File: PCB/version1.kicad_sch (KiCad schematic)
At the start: 21 parts, among them J1 USB_C_Receptacle_USB2.0_16P, SW1 SW_SPST, SW2 SW_SPST, SW3 RotaryEncoder_Switch, U1 STM32F072CBTx, U2 XC6206PxxxMR

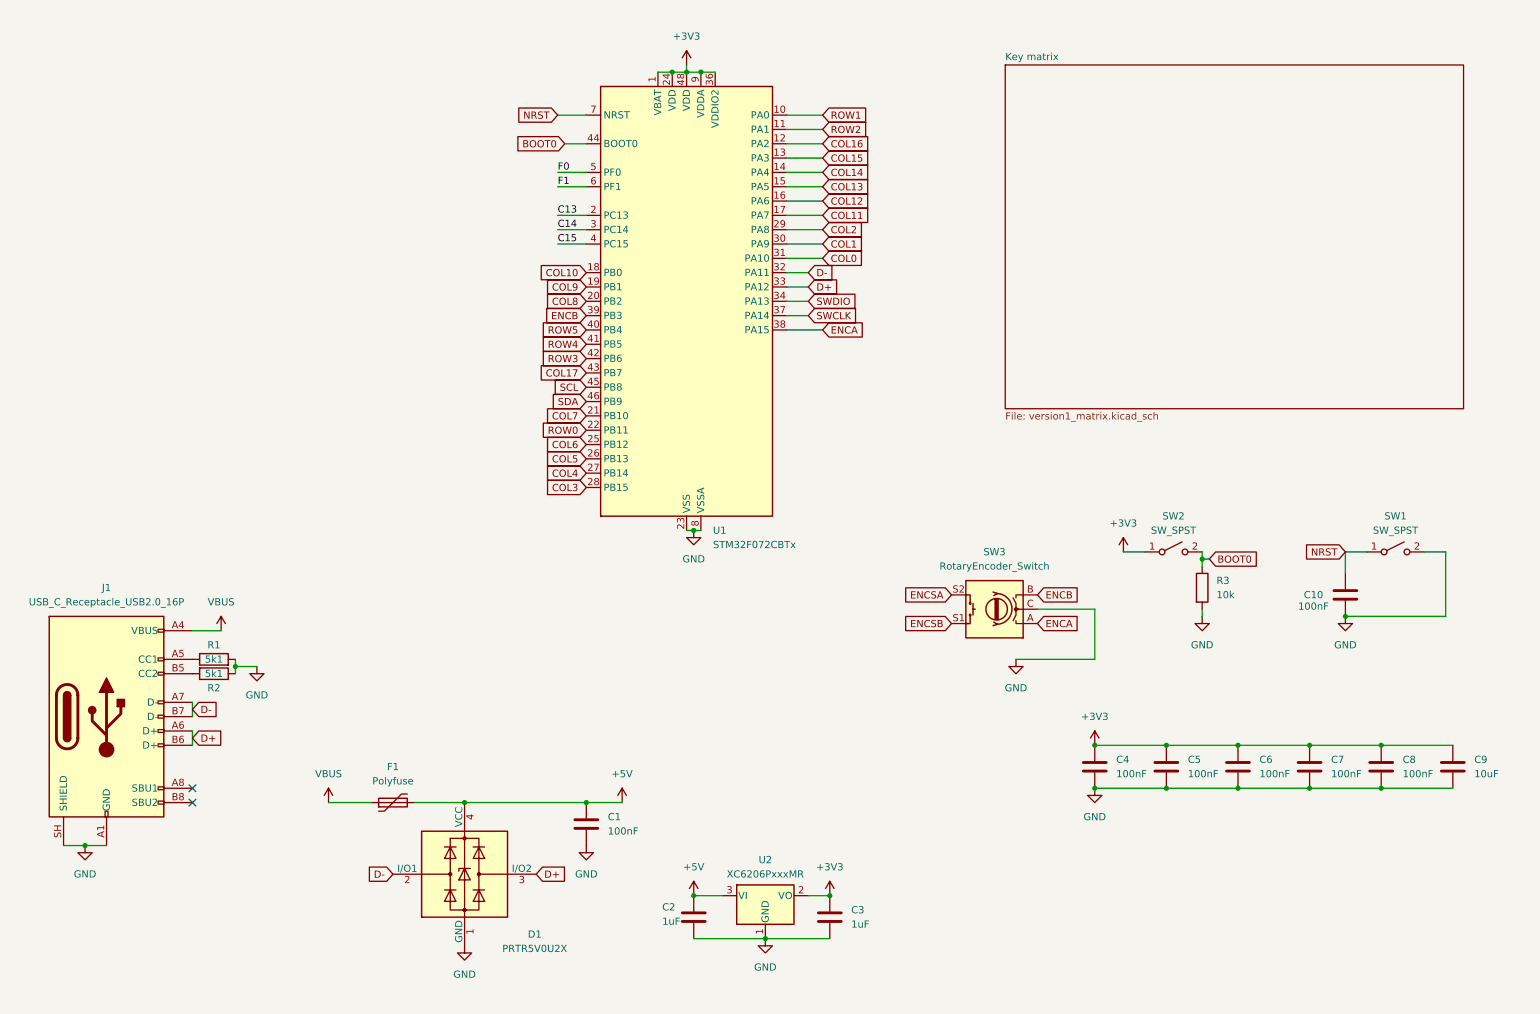
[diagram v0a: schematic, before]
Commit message: Updated schematic
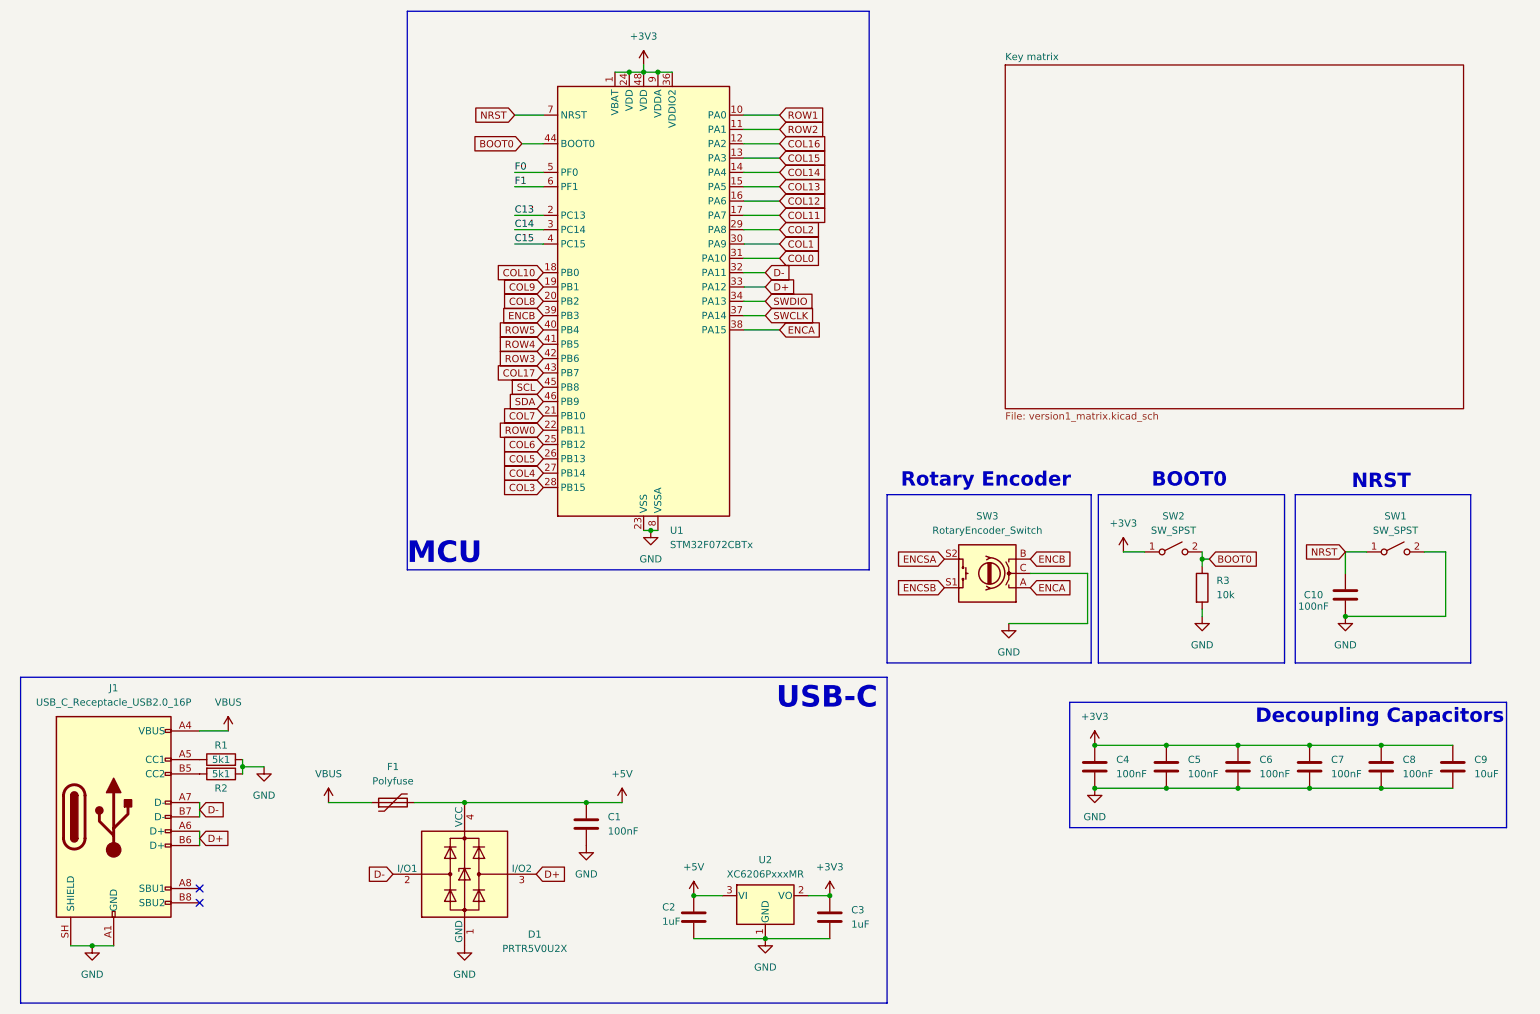
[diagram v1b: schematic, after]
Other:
- note added: "BOOT0"
- note added: "Decoupling Capacitors"
- note added: "MCU"
- note added: "NRST"
- note added: "Rotary Encoder"
- note added: "USB-C"
- moved on the sheet: J1, R1, R2, SW3, U1

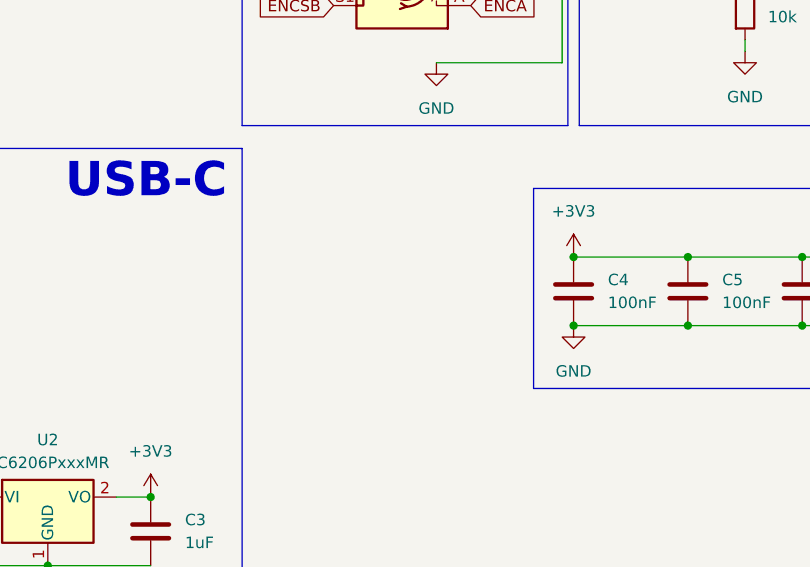
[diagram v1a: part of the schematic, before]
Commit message: Updated PCB files
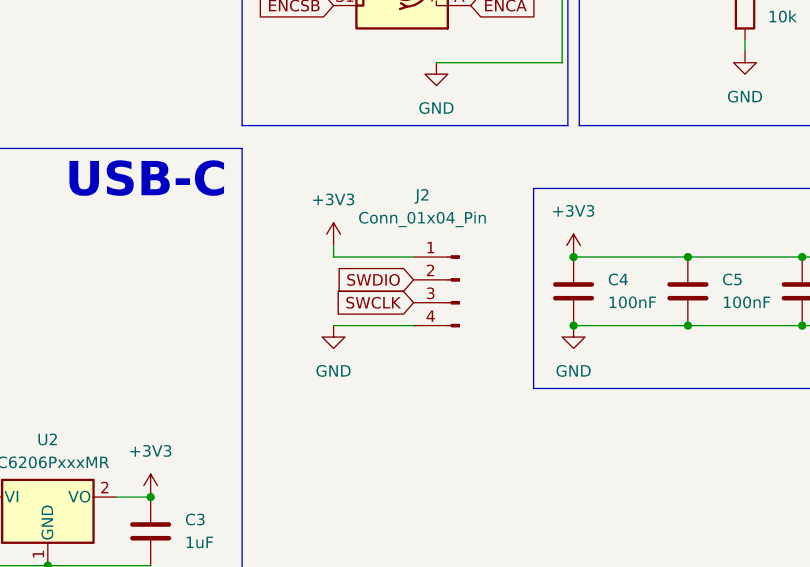
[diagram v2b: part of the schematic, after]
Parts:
- added J2: Conn_01x04_Pin, Connector_PinHeader_2.54mm:PinHeader_1x04_P2.54mm_Horizontal, symbol Connector:Conn_01x04_Pin
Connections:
- net +3V3: now also J2.1 (Pin_1)
- net GND: now also J2.4 (Pin_4)
- net SWCLK: now also J2.3 (Pin_3)
- net SWDIO: now also J2.2 (Pin_2)
